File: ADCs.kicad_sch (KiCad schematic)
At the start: 4 parts, among them U3 ADS7828, U4 ADS7828

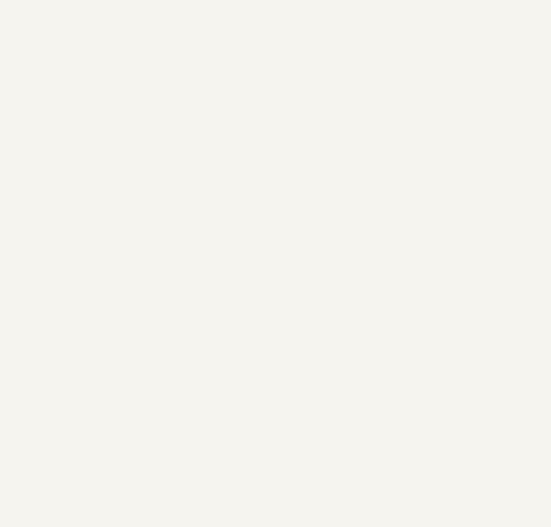
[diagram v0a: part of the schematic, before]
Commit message: added luke name
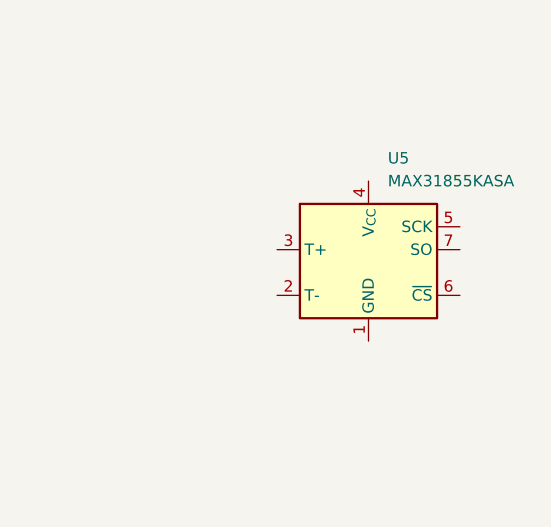
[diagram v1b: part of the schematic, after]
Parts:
- added U5: MAX31855KASA, Package_SO:SOIC-8_3.9x4.9mm_P1.27mm, symbol Sensor_Temperature:MAX31855KASA
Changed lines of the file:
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@@
+	)
+	(symbol
+		(lib_id "Sensor_Temperature:MAX31855KASA")
+		(at 185.42 48.26 0)
+		(unit 1)
+		(exclude_from_sim no)
+		(in_bom yes)
+		(on_board yes)
+		(dnp no)
+		(fields_autoplaced yes)
+		(property "Reference" "U5"
+			(at 187.5633 35.56 0)
+			(effects
+				(font
+					(size 1.27 1.27)
+				)
+				(justify left)
+			)
+		)
+		(property "Value" "MAX31855KASA"
+			(at 187.5633 38.1 0)
+			(effects
+				(font
+					(size 1.27 1.27)
+				)
+				(justify left)
+			)
+		)
+		(property "Footprint" "Package_SO:SOIC-8_3.9x4.9mm_P1.27mm"
+			(at 187.96 58.42 0)
+			(effects
+				(font
+					(size 1.27 1.27)
+					(italic yes)
+				)
+				(justify left)
+				(hide yes)
+			)
+		)
+		(property "Datasheet" "http://datasheets.maximintegrated.com/en/ds/MAX31855.pdf"
+			(at 187.96 60.96 0)
+			(effects
+				(font
+					(size 1.27 1.27)
+				)
+				(justify left)
+				(hide yes)
+			)
+		)
+		(property "Description" "Cold Junction K-type Thermocouple Interface, SPI, SOIC-8"
+			(at 187.96 55.88 0)
+			(effects
+				(font
+					(size 1.27 1.27)
+				)
+				(justify left)
+				(hide yes)
+			)
+		)
+		(pin "6"
+		)
+		(pin "4"
+		)
+		(pin "7"
+		)
+		(pin "2"
+		)
+		(pin "1"
+		)
+		(pin "5"
+		)
+		(pin "3"
+		)
+		(pin "8"
+		)
+		(instances
+			(project ""
+				(path "/bb73515c-a1ce-4448-8899-3a433fb04c26/c5809e31-49fa-4035-9e50-9a02f65a2597"
+					(reference "U5")
+					(unit 1)
+				)
+			)
+		)
 	)
 	(symbol

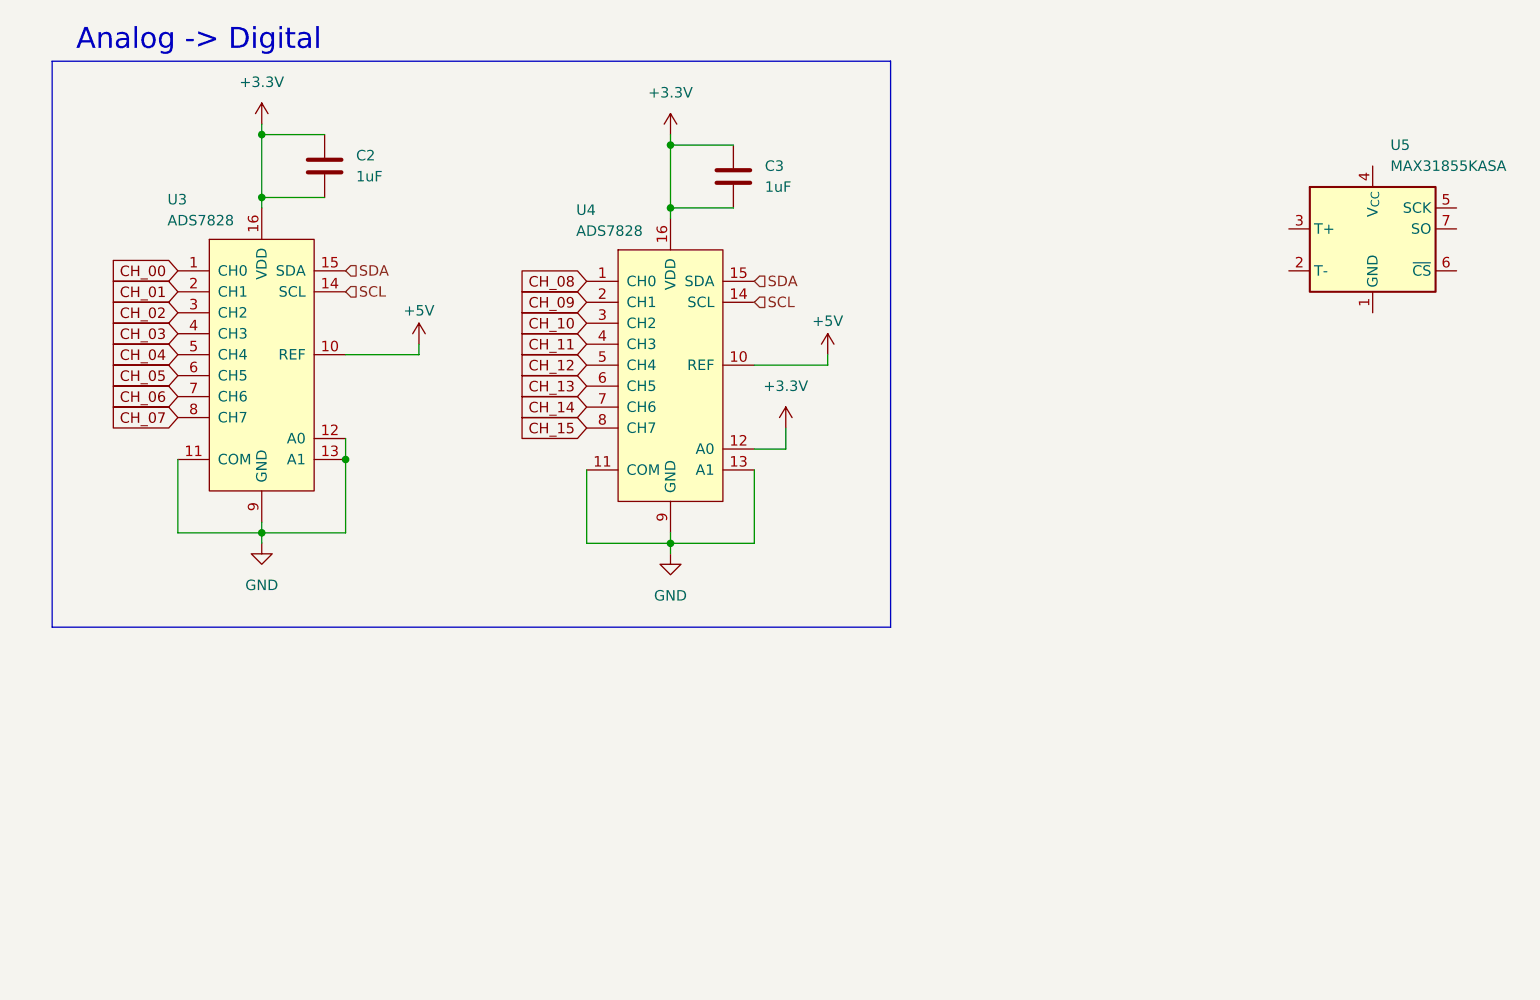
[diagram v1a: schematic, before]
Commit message: power
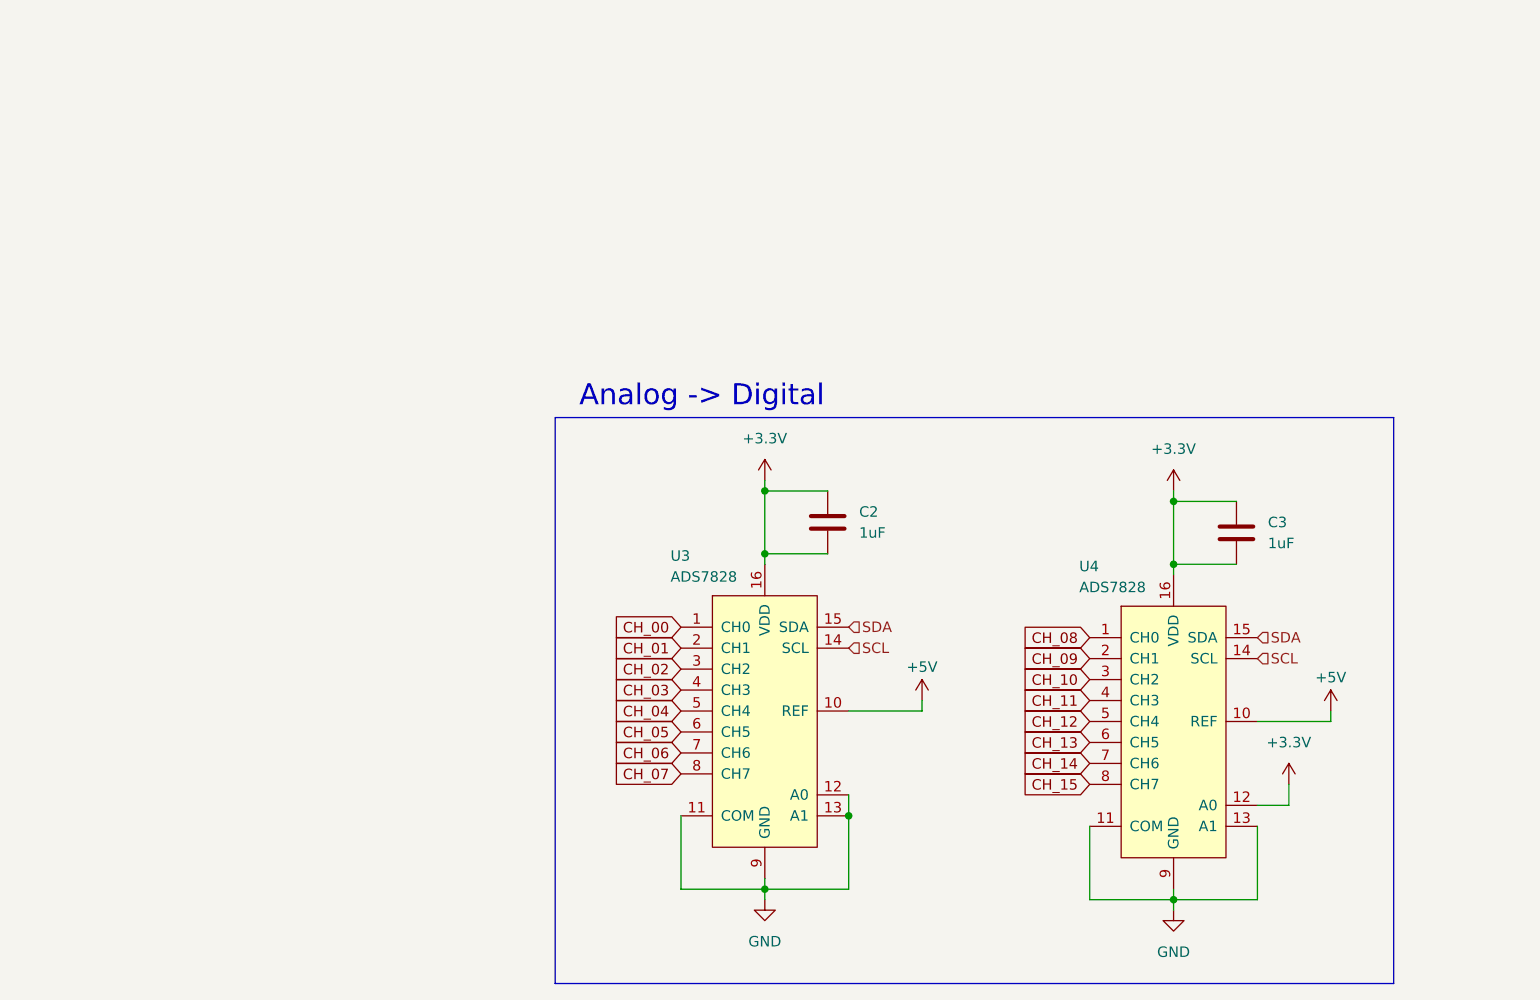
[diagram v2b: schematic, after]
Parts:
- removed U5: MAX31855KASA, Package_SO:SOIC-8_3.9x4.9mm_P1.27mm, symbol Sensor_Temperature:MAX31855KASA
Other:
- moved on the sheet: C2, C3, U3, U4
